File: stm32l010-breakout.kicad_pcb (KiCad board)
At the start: 2 copper layers, 25 x 50 mm, 30 parts, among them J1 SWD, J2 Left, J3 Right, Q1 BC847BS, SW1 Reset, U1 STM32L010K8Tx, Y1 32.768kHz

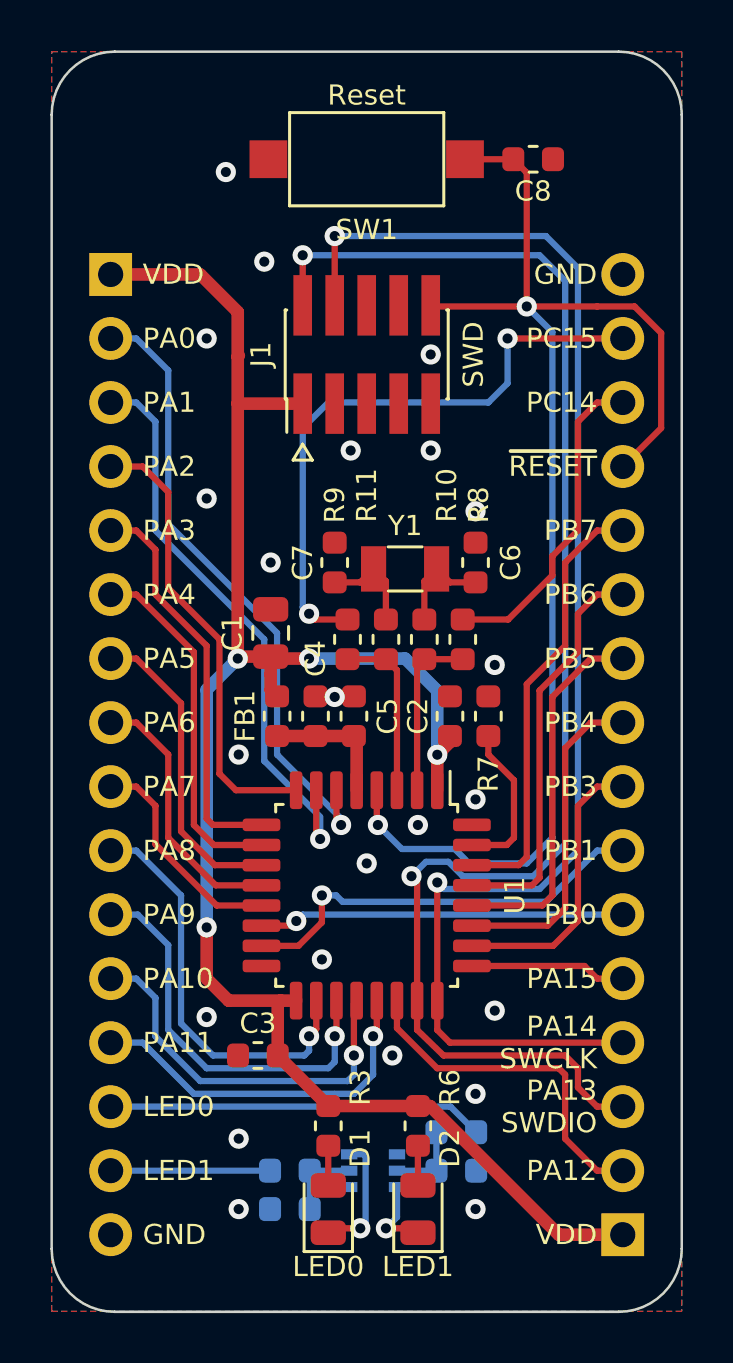
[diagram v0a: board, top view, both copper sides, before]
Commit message: Finished laying out Revision B
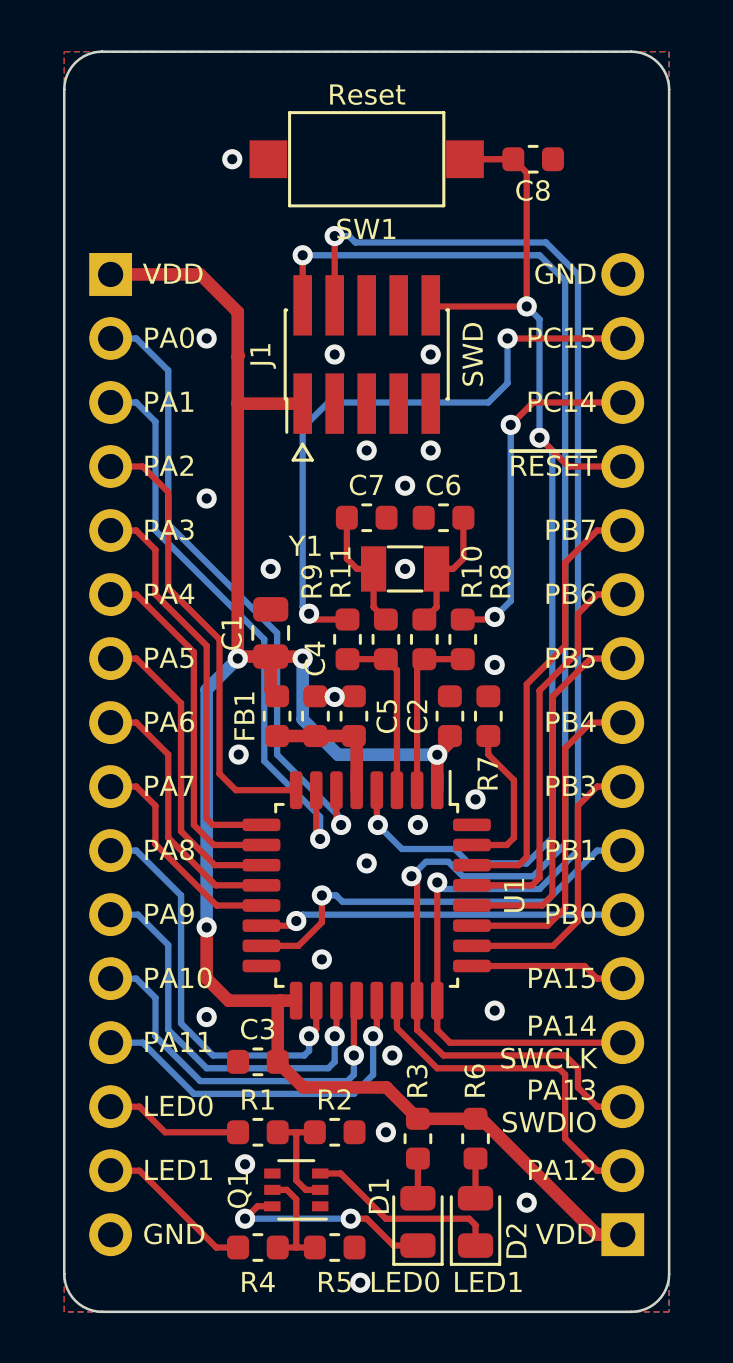
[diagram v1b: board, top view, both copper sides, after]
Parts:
- Q1: value BC847BS -> BC847CDW1; moved to F.Cu
- R1, R2, R4, R5: moved to F.Cu
- R10: value e -> 0R
- moved R1 7.87 mm to (122.7, 119.1), turned to 180 degrees
- moved R2 5.06 mm to (125.7, 119.1)
- moved D1 3.59 mm to (129.0, 122.7)
- moved R3 3.59 mm to (129.0, 119.4)
- moved R4 3.30 mm to (122.7, 123.7)
- moved Q1 3.14 mm to (124.2, 121.4)
- moved D2 2.34 mm to (131.3, 122.7)
- moved R6 2.34 mm to (131.3, 119.4)
- moved R5 2.34 mm to (125.7, 123.7), turned to 180 degrees
- moved C6 2.18 mm to (130.0, 94.7), turned to 180 degrees
- moved C7 2.18 mm to (127.0, 94.7), turned to 0 degrees
- moved C3 0.25 mm to (122.7, 116.3)
- moved #LOGO1 0.13 mm to (135.8, 80.0)
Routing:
- net /LED0: track 14.9 -> 5.48 mm
- net /~RESET: track 54.4 -> 46.5 mm, vias 2 -> 3
- net Net-(D2-Pad1): track 3.16 -> 7.82 mm, vias 1 -> 0
- net Net-(D1-Pad1): track 4.97 -> 8.59 mm, vias 1 -> 2
- net Net-(Q1-Pad2): track 3.09 -> 4.49 mm
- net Net-(Q1-Pad5): track 3.09 -> 4.49 mm
- net /PC14: track 12.9 -> 14.0 mm, vias 0 -> 2
- net Net-(C7-Pad1): track 3.97 -> 5.06 mm
- net Net-(C6-Pad1): track 3.97 -> 5.06 mm
- net GND: vias 23 -> 24
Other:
- board size 25 x 50 mm -> 24 x 50 mm
- board text removed: "JP1, JP2 settings: 1-2: PC14,PC15 connected to the Y1 crystal 2-3: PC14,PC15 connected to the J3 header"
